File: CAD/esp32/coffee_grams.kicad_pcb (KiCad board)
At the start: 2 copper layers, 81 x 99 mm, 46 parts, among them J1 USB_B_Mini, J2 Conn_01x05_Male, Q1 BC847, Q2 BC847, Q3 MMBT4403, SW1 BX_TARE, SW2 BX_ON_OFF, SW3 BX_TIMER, SW4 BX_COFFEE_G, SW5 BX_H2O_G, U1 FT232RL, U2 HX711, U3 ESP32-WROOM-32, U4 LM3940

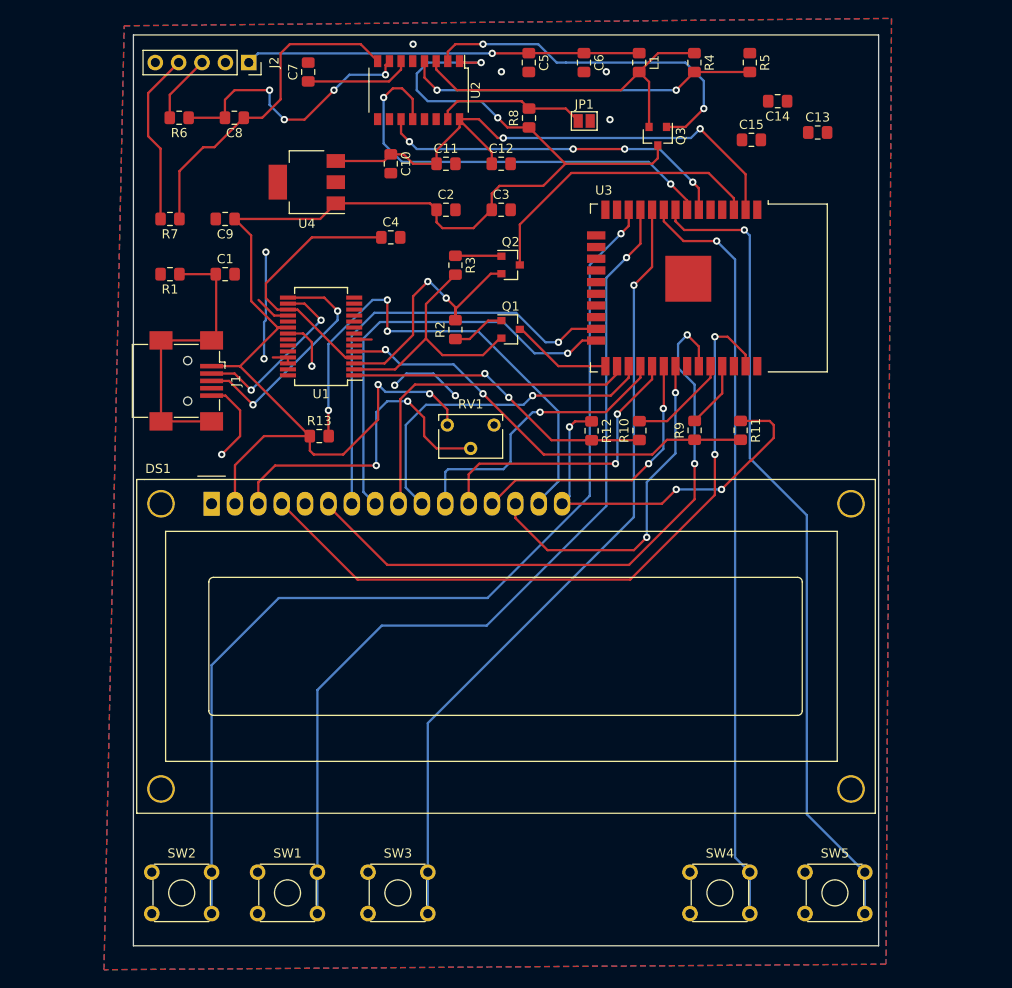
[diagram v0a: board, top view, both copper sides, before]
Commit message: pcb rev2
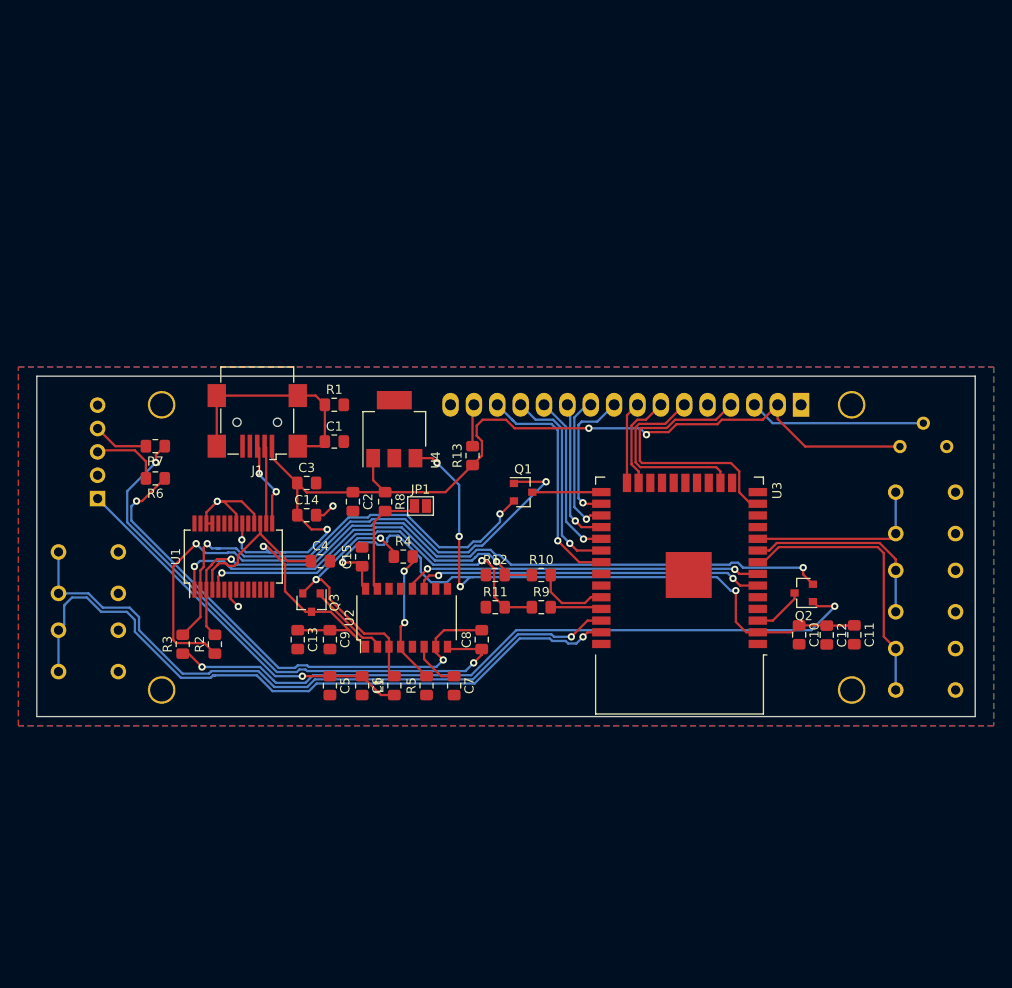
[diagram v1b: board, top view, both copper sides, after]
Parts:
- DS1, J2, RV1, SW1, SW2, SW3, SW4, SW5: moved to B.Cu
- moved C13 78.9 mm to (114.9, 123.7), turned to 270 degrees
- moved R5 76.3 mm to (128.9, 128.7), turned to 90 degrees
- moved SW3 76.1 mm to (186.4, 107.7), turned to 180 degrees
- moved L1 72.8 mm to (125.4, 128.7), turned to 90 degrees
- moved C6 71.9 mm to (121.9, 128.7)
- moved C5 71.1 mm to (118.4, 128.7)
- moved C7 68.6 mm to (131.9, 128.7), turned to 270 degrees
- moved C14 68.2 mm to (115.8, 110.2), turned to 0 degrees
- moved C10 67.8 mm to (169.4, 123.2)
- moved C11 67.8 mm to (175.4, 123.2), turned to 270 degrees
- moved DS1 65.0 mm to (169.6, 98.2), turned to 180 degrees
- moved Q3 63.1 mm to (116.4, 119.7)
- moved C8 62.8 mm to (134.9, 123.7), turned to 90 degrees
- moved R4 62.3 mm to (126.3, 114.7), turned to 0 degrees
- moved C12 62.3 mm to (172.4, 123.2), turned to 270 degrees
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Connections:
- J1 pad 4: Net-(J1-Pad4) -> (no net)
- U1 pad 10: Net-(U1-Pad10) -> (no net)
- U1 pad 11: Net-(U1-Pad11) -> (no net)
- U1 pad 12: Net-(U1-Pad12) -> (no net)
- U1 pad 13: Net-(U1-Pad13) -> (no net)
- U1 pad 14: Net-(U1-Pad14) -> (no net)
- U1 pad 19: Net-(U1-Pad19) -> (no net)
- U1 pad 22: Net-(U1-Pad22) -> (no net)
- U1 pad 23: Net-(U1-Pad23) -> (no net)
- U1 pad 27: Net-(U1-Pad27) -> (no net)
- U1 pad 28: Net-(U1-Pad28) -> (no net)
- U1 pad 6: Net-(U1-Pad6) -> (no net)
- U1 pad 9: Net-(U1-Pad9) -> (no net)
- U2 pad 10: Net-(U2-Pad10) -> (no net)
- U2 pad 13: Net-(U2-Pad13) -> (no net)
- U2 pad 9: Net-(U2-Pad9) -> (no net)
- U3 pad 11: /BX_TARE -> (no net)
- U3 pad 12: /BX_ON_OFF -> (no net)
- U3 pad 13: Net-(U3-Pad13) -> /LCD_RS
- U3 pad 14: Net-(U3-Pad14) -> (no net)
- U3 pad 16: Net-(U3-Pad16) -> /LCD_E
- U3 pad 17: Net-(U3-Pad17) -> (no net)
- U3 pad 18: Net-(U3-Pad18) -> (no net)
- U3 pad 19: Net-(U3-Pad19) -> (no net)
- U3 pad 20: Net-(U3-Pad20) -> (no net)
- U3 pad 21: Net-(U3-Pad21) -> (no net)
- U3 pad 22: Net-(U3-Pad22) -> (no net)
- U3 pad 32: Net-(U3-Pad32) -> (no net)
- U3 pad 33: /LCD_E -> (no net)
- U3 pad 36: Net-(U3-Pad36) -> /BX_TARE
- U3 pad 37: /LCD_RS -> /BX_ON_OFF
- U3 pad 4: Net-(U3-Pad4) -> (no net)
- U3 pad 5: Net-(U3-Pad5) -> (no net)
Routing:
- net Net-(Q2-Pad1): track 5.02 -> 78.2 mm, vias 0 -> 2
- net GND: track 85.4 -> 16.9 mm, vias 13 -> 3
- net /BX_TIMER: track 86.6 -> 19.7 mm, vias 1 -> 0
- net /BX_COFFEE_G: track 82.5 -> 21.8 mm, vias 1 -> 0
- net Net-(Q1-Pad1): track 5.83 -> 65.6 mm, vias 0 -> 2
- net /BX_H2O_G: track 88.8 -> 30.1 mm, vias 1 -> 0
- net /RTS: track 27.5 -> 79.9 mm
- net Net-(DS1-Pad15): track 55.7 -> 4.56 mm, vias 3 -> 0
- net /LCD_E: track 68.6 -> 21.0 mm, vias 2 -> 0
- net /LCD_RS: track 76.9 -> 30.6 mm, vias 2 -> 0
- net /LCD_D1: track 46.5 -> 8.96 mm, vias 1 -> 0
- net /LCD_D0: track 47.8 -> 10.7 mm, vias 1 -> 0
- net /BX_ON_OFF: track 108.6 -> 74.5 mm
- net Net-(Q3-Pad1): track 38.7 -> 8.96 mm, vias 2 -> 0
- net +3V3: track 62.1 -> 89.2 mm, vias 2 -> 5
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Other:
- board size 81 x 99 mm -> 102 x 37 mm
- board text added: "A+"
- board text added: "A-"
- board text added: "E+"
- board text added: "E-"
- board text added: "Shield"
- board text removed: "Coffee Grams Enoch Chau 2020"
